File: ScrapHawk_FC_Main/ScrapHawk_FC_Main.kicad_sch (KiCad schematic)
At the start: 48 parts, among them IC1 MP1584EN-LF-Z, J1 USB_C_Receptacle_USB2.0_16P, J2 Conn_01x06, U1 RP2040, U2 W25Q128JVS, U3 AMS1117CD-3.3, U4 LSM6DS3TR, Y1 12M

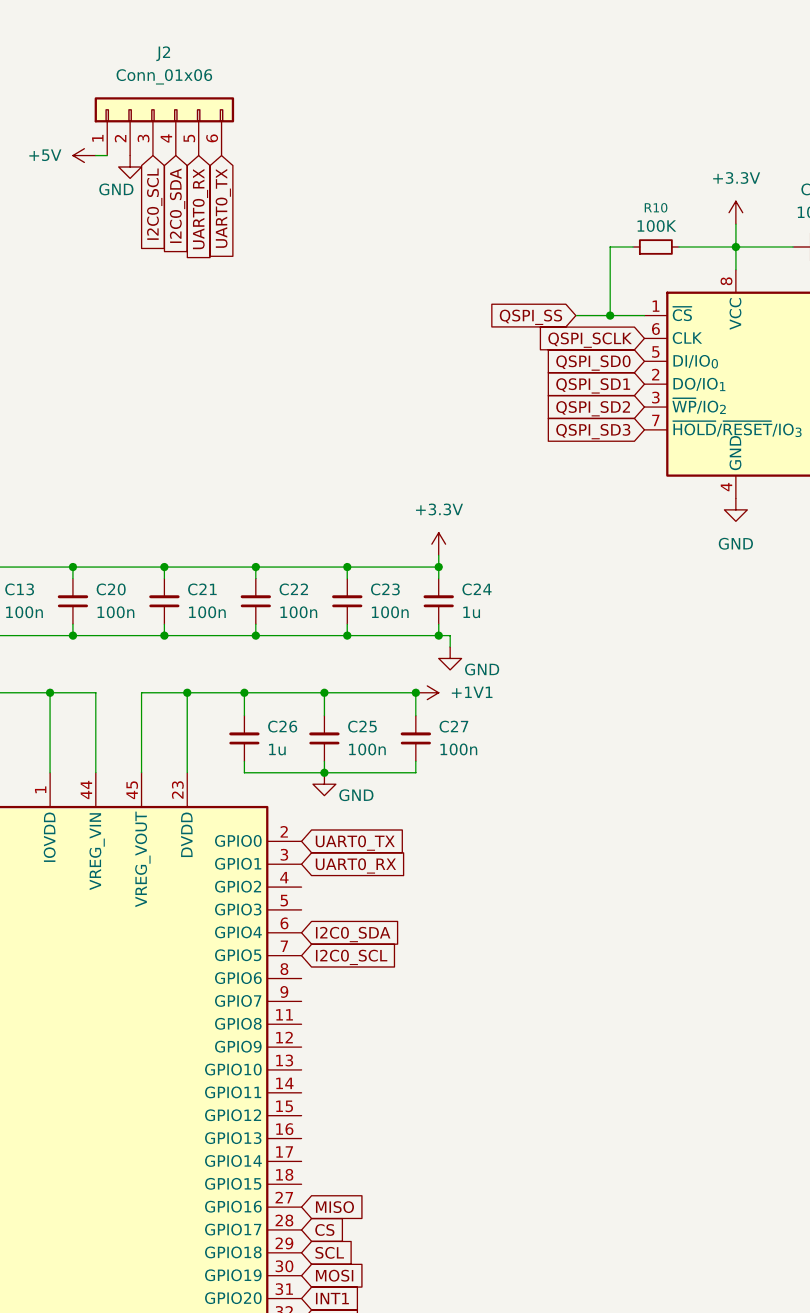
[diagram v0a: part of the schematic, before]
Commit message: finish pcb wiring
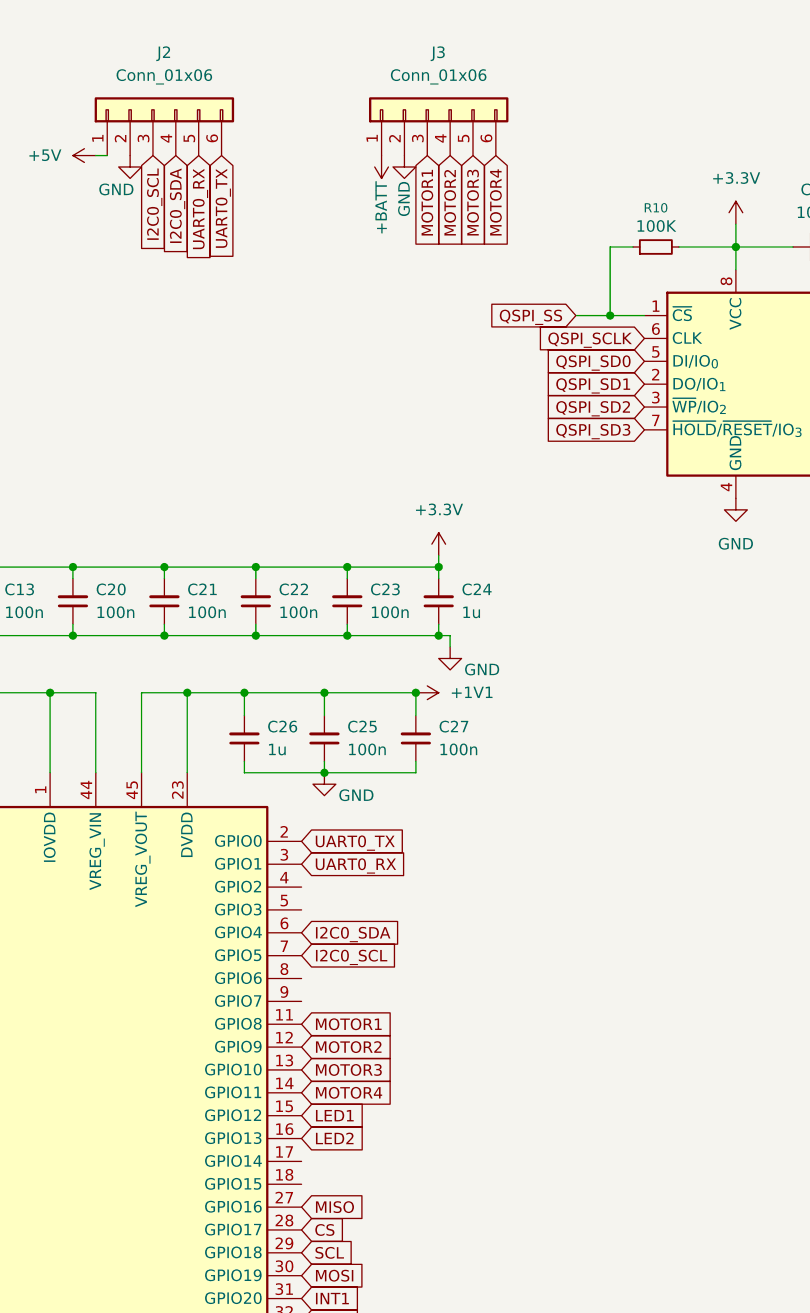
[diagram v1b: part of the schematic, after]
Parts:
- added J3: Conn_01x06, Connector_JST:JST_SH_BM06B-SRSS-TB_1x06-1MP_P1.00mm_Vertical, symbol Connector_Generic:Conn_01x06
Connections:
- net +BATT: now also J3.1 (Pin_1)
- net GND: now also J3.2 (Pin_2)
- net LED1: now also U1.15 (GPIO12)
- net LED2: now also U1.16 (GPIO13)
- net MOTOR1: now reaches U1.11 (GPIO8)
- net MOTOR1: now also J3.3 (Pin_3)
- net MOTOR2: now reaches U1.12 (GPIO9)
- net MOTOR2: now also J3.4 (Pin_4)
- net MOTOR3: now reaches U1.13 (GPIO10)
- net MOTOR3: now also J3.5 (Pin_5)
- net MOTOR4: now reaches U1.14 (GPIO11)
- net MOTOR4: now also J3.6 (Pin_6)
